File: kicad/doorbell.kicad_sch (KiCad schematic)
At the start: 107 parts, among them J1 USB-JST, J2 WF26 bus, K1 GAQW212GS, K2 GAQY212GS, K3 GAQY412EH, K4 GAQY412EH, K5 G6K-2F-Y DC12, K6 GAQY412EH, Q3 AO3400A, Q4 AO3400A, SW1 BOOT, SW2 EN, SW3 Tueroeffner (door release), SW4 Sprechen/Hoeren (talk), U1 ESP32-S3-WROOM-1U-N16R8, U2 SGM2212-3.3, U3 ES8311, U4 LP5907MFX-3.3

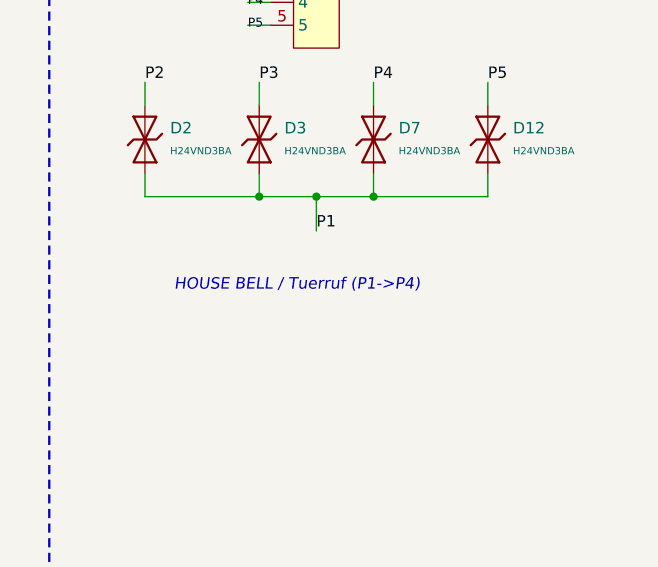
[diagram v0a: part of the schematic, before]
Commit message: Derisk V4.2 hardware changes
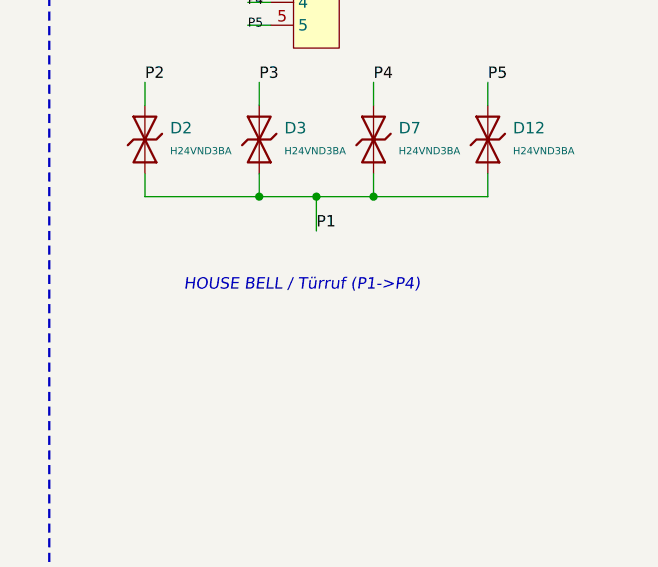
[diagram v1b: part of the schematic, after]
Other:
- note added: "HOUSE BELL / Türruf (P1->P4)"
- note removed: "HOUSE BELL / Tuerruf (P1->P4)"
